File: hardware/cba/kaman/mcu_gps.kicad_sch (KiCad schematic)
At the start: 40 parts, among them Q1 MMDT5551, Q2 DTC143X, Q3 DTC143X, SW1 SW_Push, SW2 SW_Push, U1 ESP32-C6-MINI-1, U2 L80-R, U3 NEO-M8N, U4 AT24CS64-SSHM

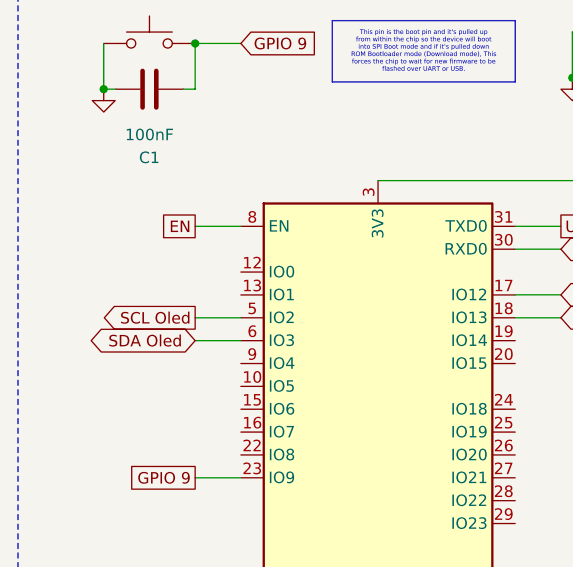
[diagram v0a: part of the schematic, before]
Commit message: hw(pcb): unorganized overlay 0.1v pcb
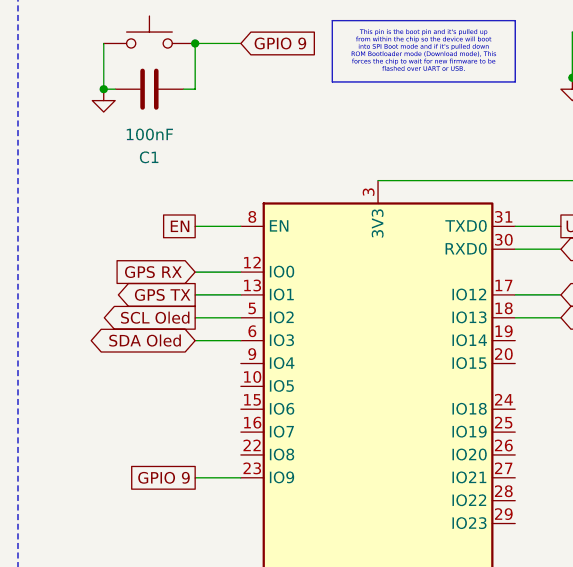
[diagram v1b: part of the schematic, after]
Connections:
- net GPS RX: now also U1.12 (IO0)
- net GPS TX: now also U1.13 (IO1)
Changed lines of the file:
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@@
+	(wire
+		(pts
+			(xy 31.75 82.55) (xy 36.83 82.55)
+		)
+		(stroke
+			(width 0)
+			(type default)
+		)
+	)
 	(wire
 		(pts
@@
 		(pts
 			(xy 144.78 27.94) (xy 157.48 27.94)
+		)
+		(stroke
+			(width 0)
+			(type default)
+		)
+	)
+	(wire
+		(pts
+			(xy 31.75 85.09) (xy 36.83 85.09)
 		)
 		(stroke
@@
 		)
 	)
+	(global_label "GPS RX"
+		(shape input)
+		(at 31.75 82.55 180)
+		(fields_autoplaced yes)
+		(effects
+			(font
+				(size 1.27 1.27)
+			)
+			(justify right)
+		)
+		(property "Intersheetrefs" "${INTERSHEET_REFS}"
+			(at 21.5682 82.55 0)
+			(hide yes)
+			(show_name no)
+			(do_not_autoplace no)
+			(effects
+				(font
+					(size 1.27 1.27)
+				)
+				(justify right)
+			)
+		)
+	)
 	(global_label "UART RX"
 		(shape input)
@@
 			(hide yes)
 			(show_name no)
+			(do_not_autoplace no)
+			(effects
+				(font
+					(size 1.27 1.27)
+				)
+				(justify right)
+			)
+		)
+	)
+	(global_label "GPS TX"
+		(shape output)
+		(at 31.75 85.09 180)
+		(fields_autoplaced yes)
+		(effects
+			(font
+				(size 1.27 1.27)
+			)
+			(justify right)
+		)
+		(property "Intersheetrefs" "${INTERSHEET_REFS}"
+			(at 21.8706 85.09 0)
+			(hide yes)
+			(show_name no)
